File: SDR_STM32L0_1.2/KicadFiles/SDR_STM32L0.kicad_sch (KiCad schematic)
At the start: 24 parts, among them SW1 SW_SPDT, U3 STM32L010RBTx, U4 AMS1117-3.3, Y1 32 MHz

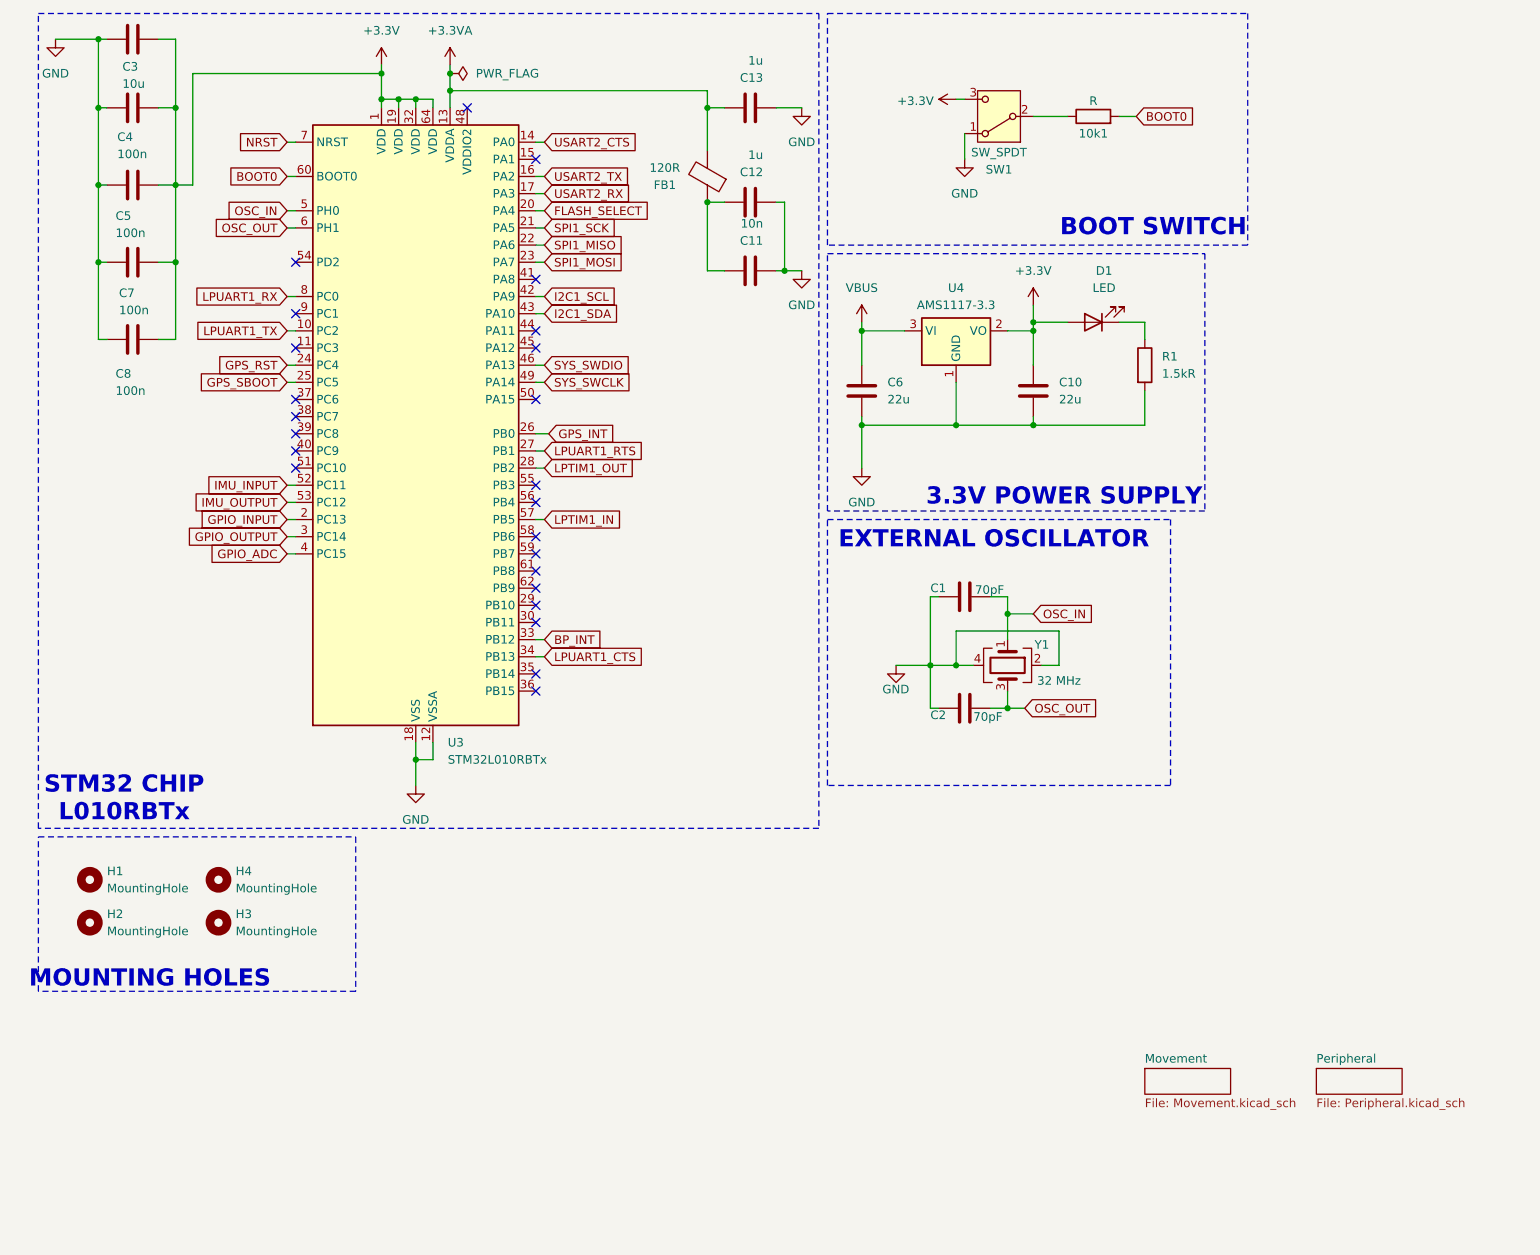
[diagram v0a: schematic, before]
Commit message: dev
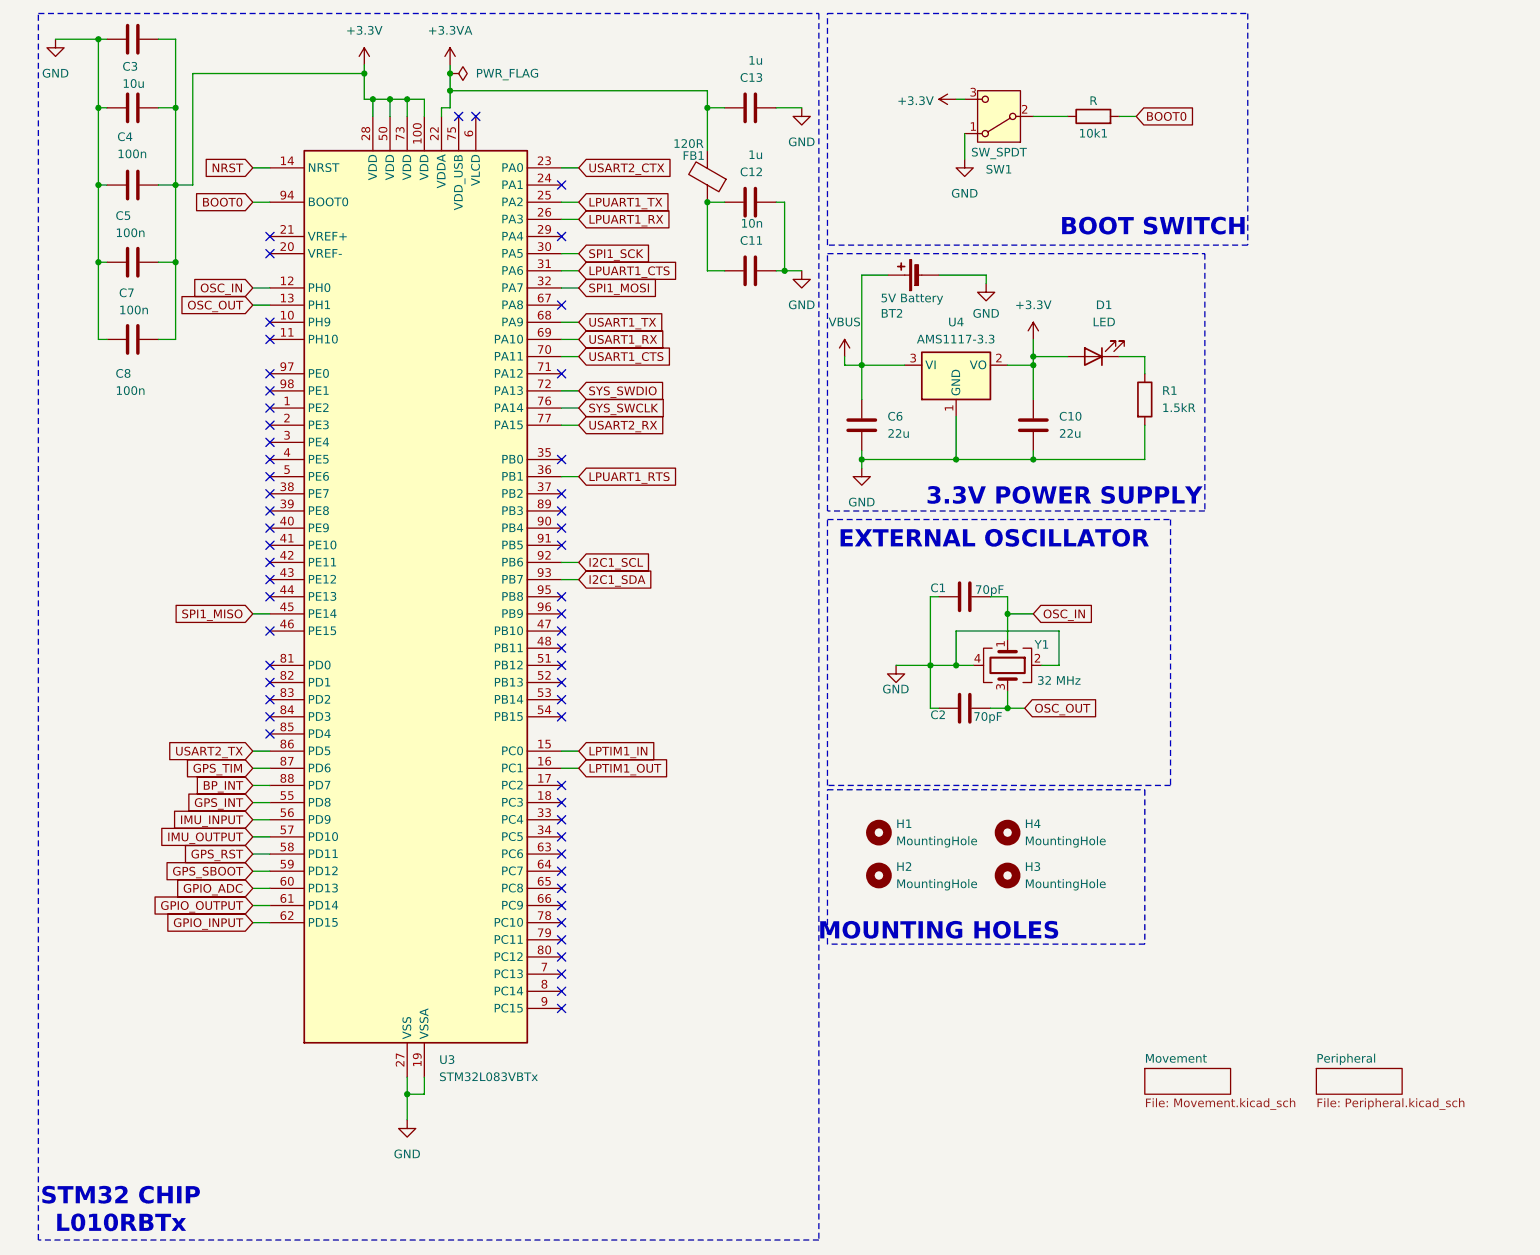
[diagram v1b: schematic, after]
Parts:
- removed U3: STM32L010RBTx, Package_QFP:LQFP-64_10x10mm_P0.5mm, symbol MCU_ST_STM32L0:STM32L010RBTx
- added BT2: 5V Battery, symbol Device:Battery_Cell
- added U3: STM32L083VBTx, Package_QFP:LQFP-100_14x14mm_P0.5mm, symbol MCU_ST_STM32L0:STM32L083VBTx
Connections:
- net +3.3V: now also U3.100 (VDD), U3.28 (VDD), U3.50 (VDD), U3.73 (VDD)
- net +3.3VA: now also U3.22 (VDDA)
- net BOOT0: now also U3.94 (BOOT0)
- net BP_INT: now also U3.88 (PD7)
- net GND: now also BT2.2 (-), U3.19 (VSSA), U3.27 (VSS), U3.49 (VSS), U3.74 (VSS), U3.99 (VSS)
- net GPIO_ADC: now also U3.60 (PD13)
- net GPIO_INPUT: now also U3.62 (PD15)
- net GPIO_OUTPUT: now also U3.61 (PD14)
- net GPS_INT: now also U3.55 (PD8)
- net GPS_RST: now also U3.58 (PD11)
- net GPS_SBOOT: now also U3.59 (PD12)
- net I2C1_SCL: now also U3.92 (PB6)
- net I2C1_SDA: now also U3.93 (PB7)
- net IMU_INPUT: now also U3.56 (PD9)
- net IMU_OUTPUT: now also U3.57 (PD10)
- net LPTIM1_IN: now also U3.15 (PC0)
- net LPTIM1_OUT: now also U3.16 (PC1)
- net LPUART1_CTS: now also U3.31 (PA6)
- net LPUART1_RTS: now also U3.36 (PB1)
- net LPUART1_RX: now also U3.26 (PA3)
- net LPUART1_TX: now also U3.25 (PA2)
- net NRST: now also U3.14 (NRST)
- net OSC_IN: now also U3.12 (PH0)
- net OSC_OUT: now also U3.13 (PH1)
- net SPI1_MISO: now also U3.45 (PE14)
- net SPI1_MOSI: now also U3.32 (PA7)
- net SPI1_SCK: now also U3.30 (PA5)
- net SYS_SWCLK: now also U3.76 (PA14)
- net SYS_SWDIO: now also U3.72 (PA13)
- net USART2_RX: now also U3.77 (PA15)
- net USART2_TX: now also U3.86 (PD5)
- net VBUS: now also BT2.1 (+)
- new net GPS_TIM: U3.87 (PD6)
- new net USART1_CTS: U3.70 (PA11)
- new net USART1_RX: U3.69 (PA10)
- new net USART1_TX: U3.68 (PA9)
- new net USART2_CTX: U3.23 (PA0)
- no-connect marks 24 -> 57
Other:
- moved on the sheet: C10, C6, D1, H1, H2, H3, H4, R1, U4

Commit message: added 1.2 back
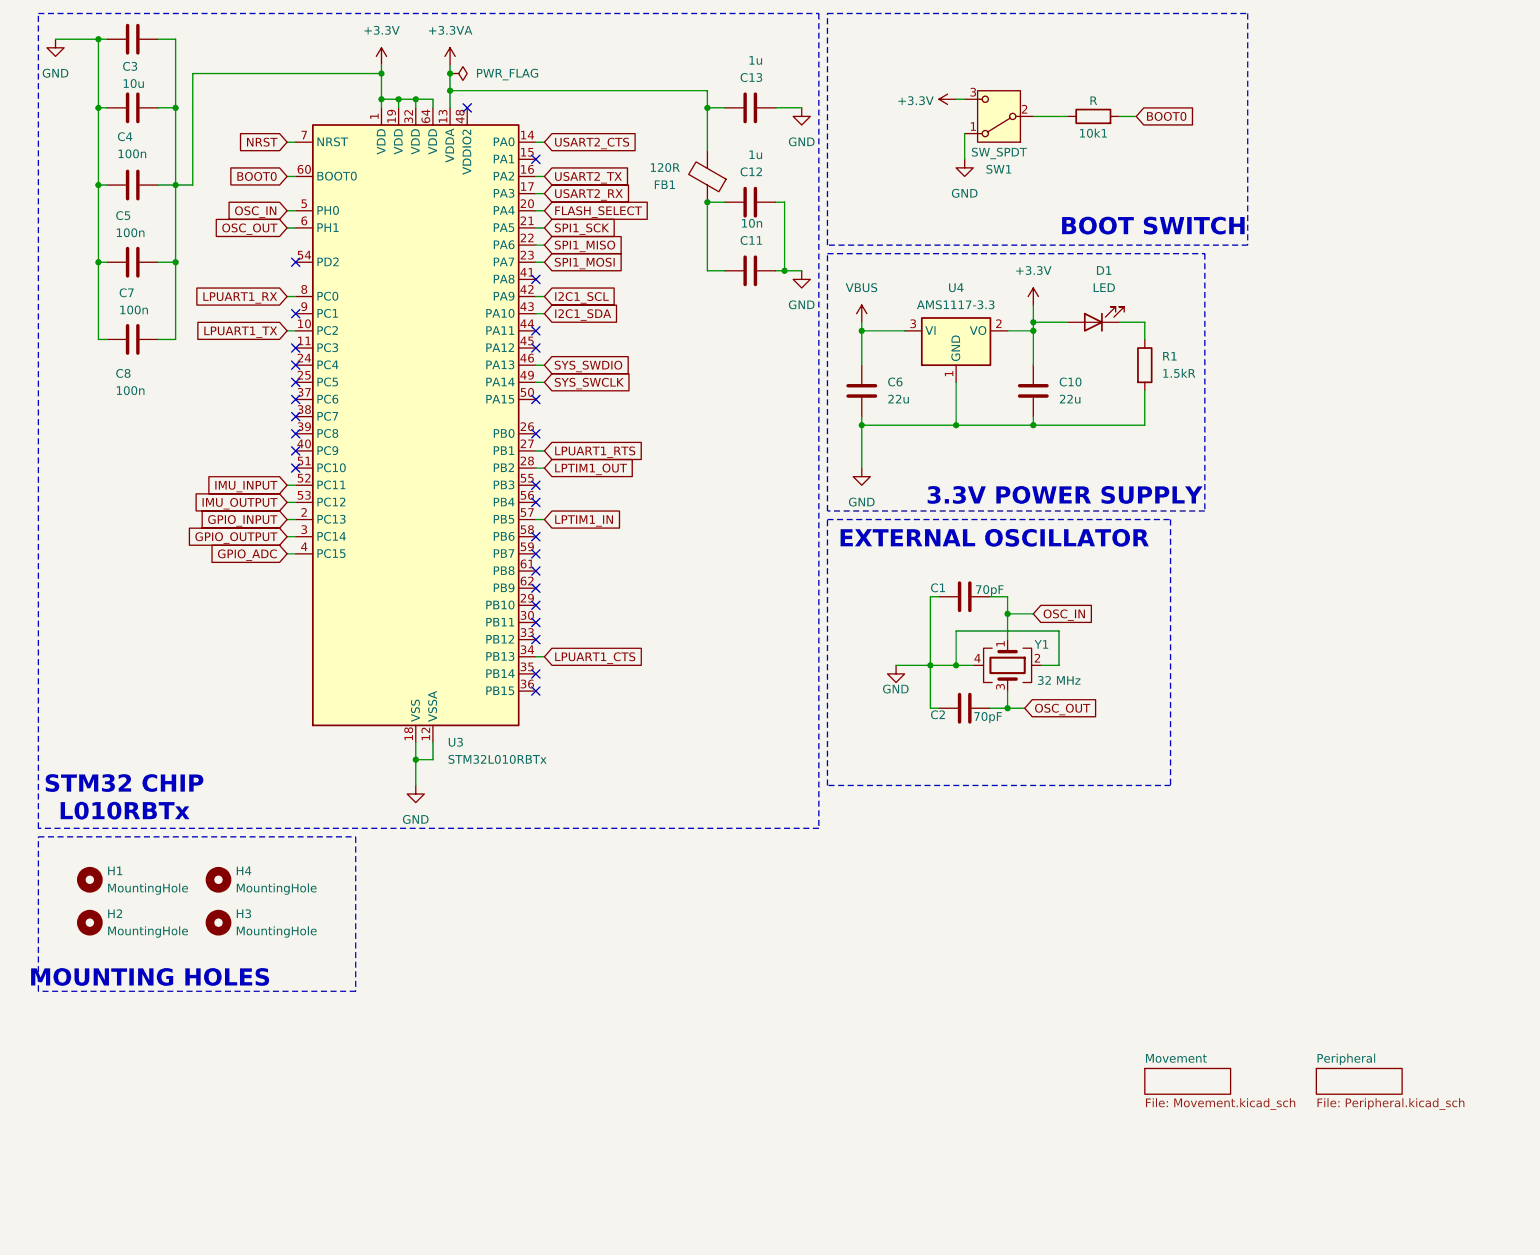
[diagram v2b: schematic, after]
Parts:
- removed BT2: 5V Battery, symbol Device:Battery_Cell
- removed U3: STM32L083VBTx, Package_QFP:LQFP-100_14x14mm_P0.5mm, symbol MCU_ST_STM32L0:STM32L083VBTx
- added U3: STM32L010RBTx, Package_QFP:LQFP-64_10x10mm_P0.5mm, symbol MCU_ST_STM32L0:STM32L010RBTx
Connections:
- net +3.3V: now also U3.1 (VDD), U3.19 (VDD), U3.32 (VDD), U3.64 (VDD)
- net +3.3VA: now also U3.13 (VDDA)
- net BOOT0: now also U3.60 (BOOT0)
- net GND: now also U3.12 (VSSA), U3.18 (VSS), U3.31 (VSS), U3.47 (VSS), U3.63 (VSS)
- net GPIO_ADC: now also U3.4 (PC15)
- net GPIO_INPUT: now also U3.2 (PC13)
- net GPIO_OUTPUT: now also U3.3 (PC14)
- net I2C1_SCL: now also U3.42 (PA9)
- net I2C1_SDA: now also U3.43 (PA10)
- net IMU_INPUT: now also U3.52 (PC11)
- net IMU_OUTPUT: now also U3.53 (PC12)
- net LPTIM1_IN: now also U3.57 (PB5)
- net LPTIM1_OUT: now also U3.28 (PB2)
- net LPUART1_CTS: now also U3.34 (PB13)
- net LPUART1_RTS: now also U3.27 (PB1)
- net LPUART1_RX: now also U3.8 (PC0)
- net LPUART1_TX: now also U3.10 (PC2)
- net NRST: now also U3.7 (NRST)
- net OSC_IN: now also U3.5 (PH0)
- net OSC_OUT: now also U3.6 (PH1)
- net SPI1_MISO: now also U3.22 (PA6)
- net SPI1_MOSI: now also U3.23 (PA7)
- net SPI1_SCK: now also U3.21 (PA5)
- net SYS_SWCLK: now also U3.49 (PA14)
- net SYS_SWDIO: now also U3.46 (PA13)
- net USART2_RX: now also U3.17 (PA3)
- net USART2_TX: now also U3.16 (PA2)
- new net FLASH_SELECT: U3.20 (PA4)
- new net USART2_CTS: U3.14 (PA0)
- no-connect marks 57 -> 28
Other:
- moved on the sheet: C10, C6, D1, H1, H2, H3, H4, R1, U4
